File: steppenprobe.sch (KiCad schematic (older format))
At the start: 84 parts, among them J1 USB_C_Receptacle_USB2.0, J2 Conn_ST_STDC14, J4 Conn_01x16, Q1 2N7002, SW1 SW_SPDT, SW2 SW_Push, U1 FT2232H, U10 74LVC1G125, U11 74LVC1G125, U12 74LVC1G125, U2 XC6206PxxxMR, U3 SRV05-4, U4 93LCxxB, U5 74LVC1G125, U6 74LVC1G126, U7 74LVC1G125, U8 74LVC1G125, U9 74LVC1G125, Y1 Crystal_GND24

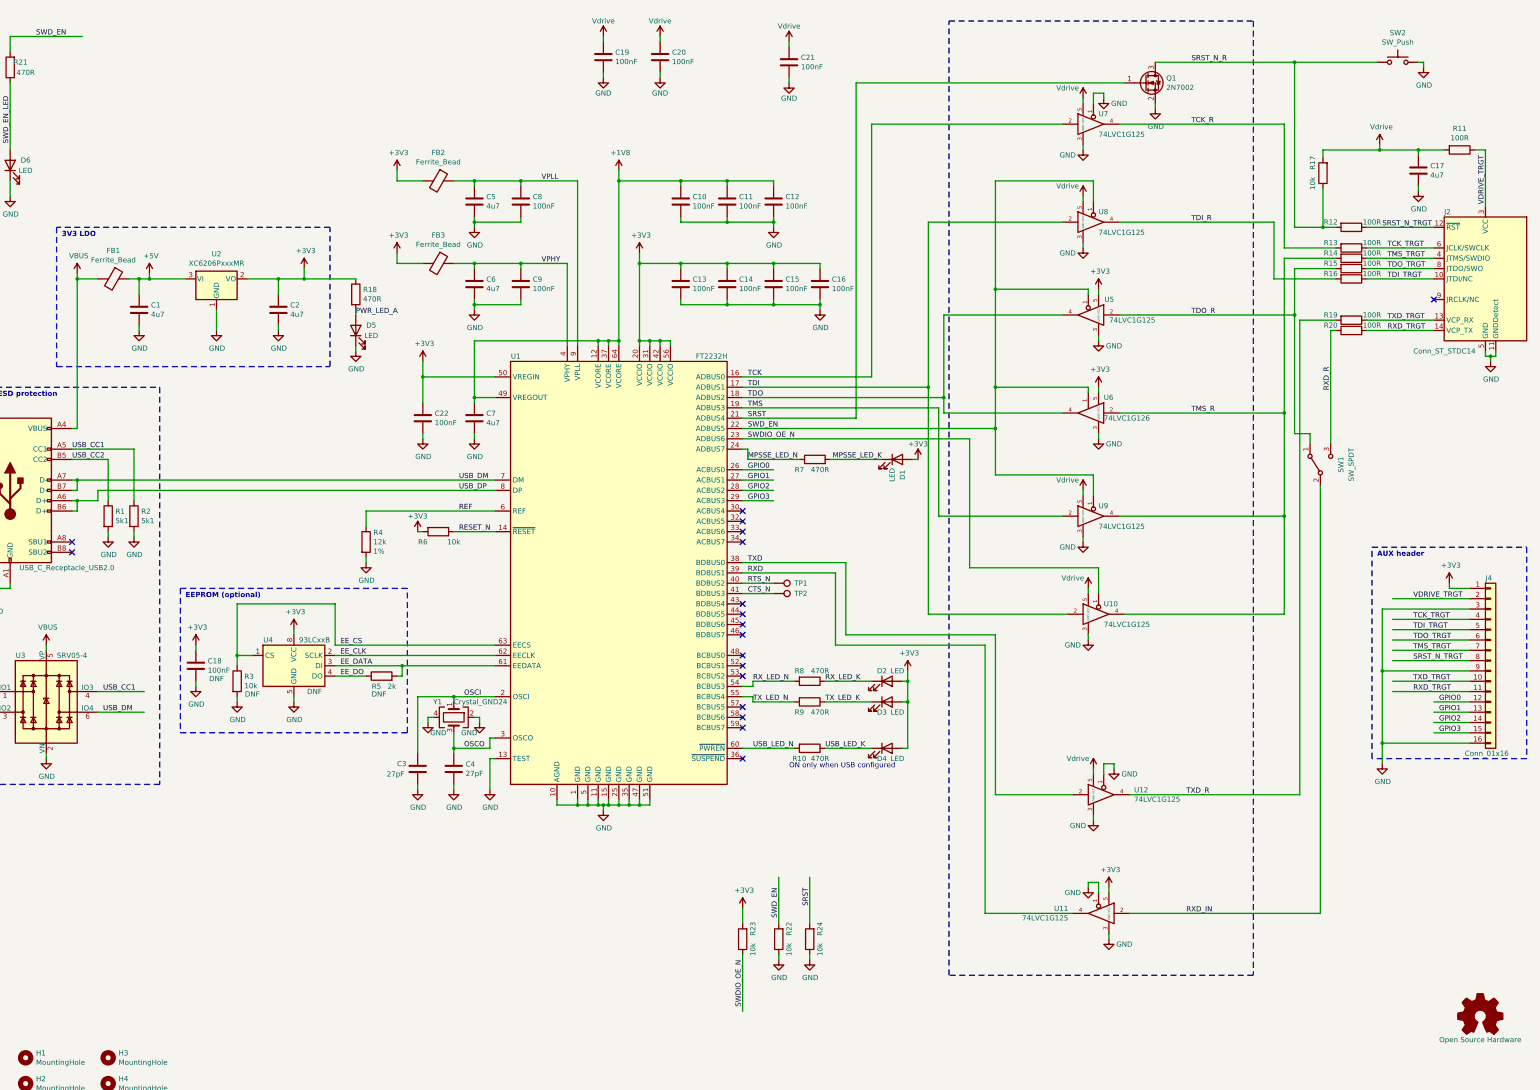
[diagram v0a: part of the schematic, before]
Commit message: Tidy-up schematic.
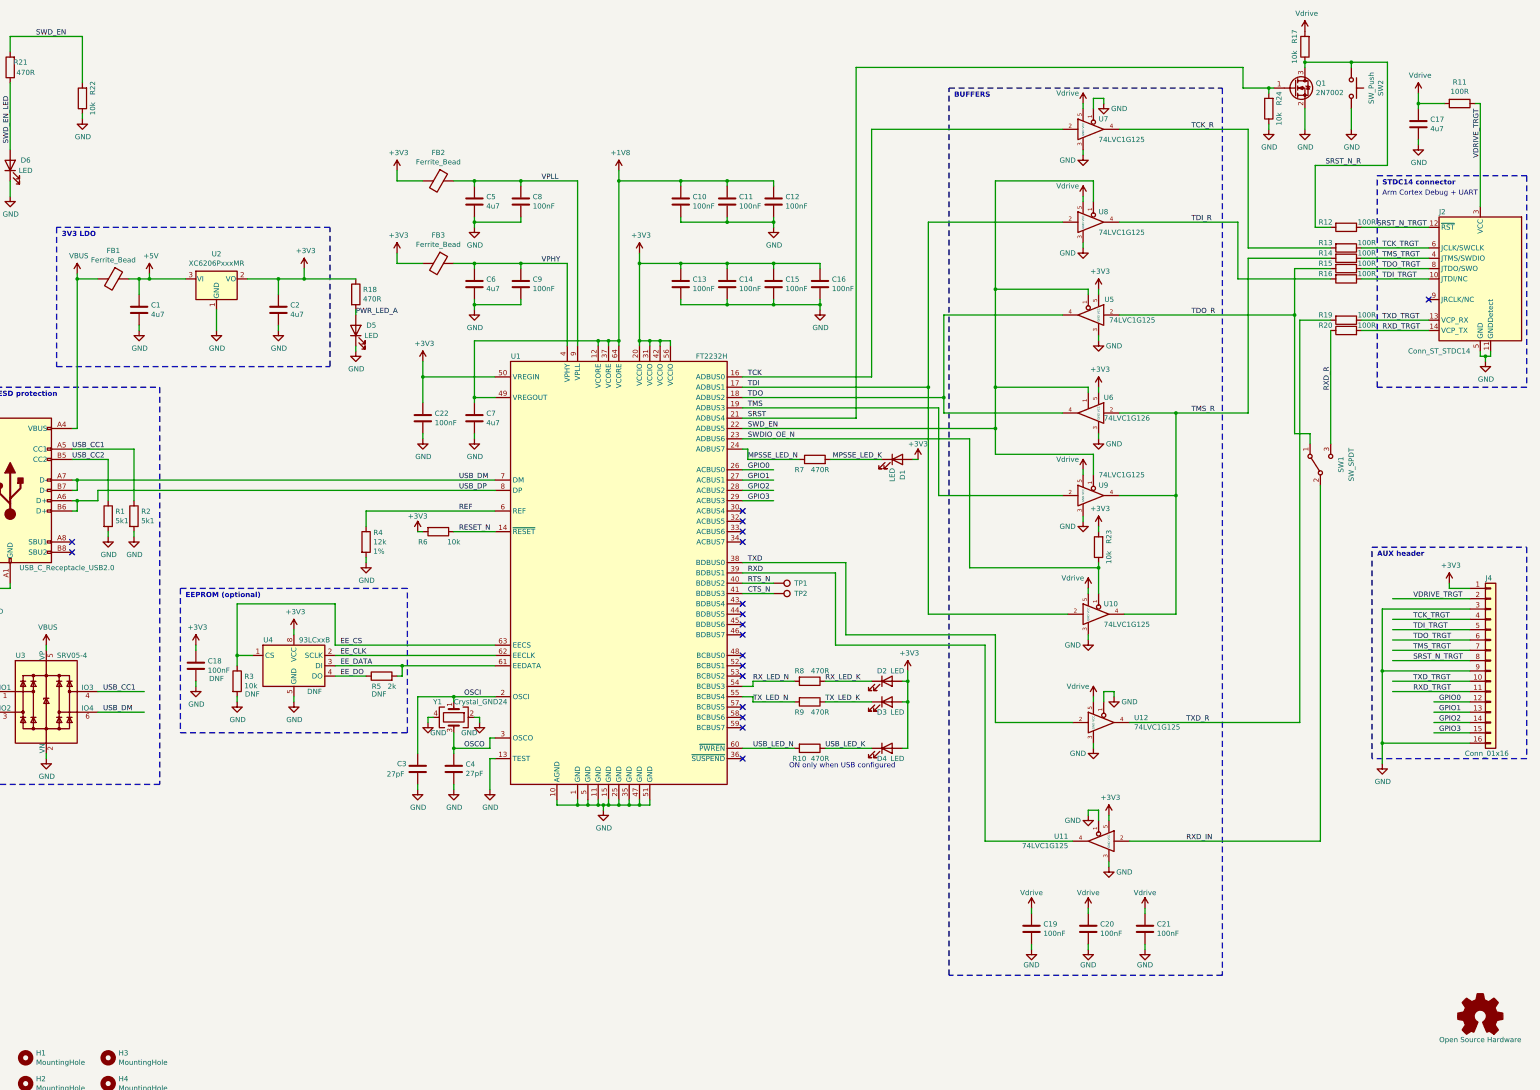
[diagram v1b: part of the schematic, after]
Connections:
- wire segments 371 -> 372
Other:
- note added: "Arm Cortex Debug + UART"
- note added: "BUFFERS"
- note added: "STDC14 connector"
- moved on the sheet: C17, C19, C20, C21, J2, Q1, R11, R12, R13, R14, R15, R16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
